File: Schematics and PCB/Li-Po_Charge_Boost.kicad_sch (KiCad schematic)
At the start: 29 parts, among them Q1 FS8205, SW107 Battery Switch, U19 TLV71311PDBVR, U20 TLV70033DDCR, U7 TP4056, U8 MT3608, U9 FS312F-G

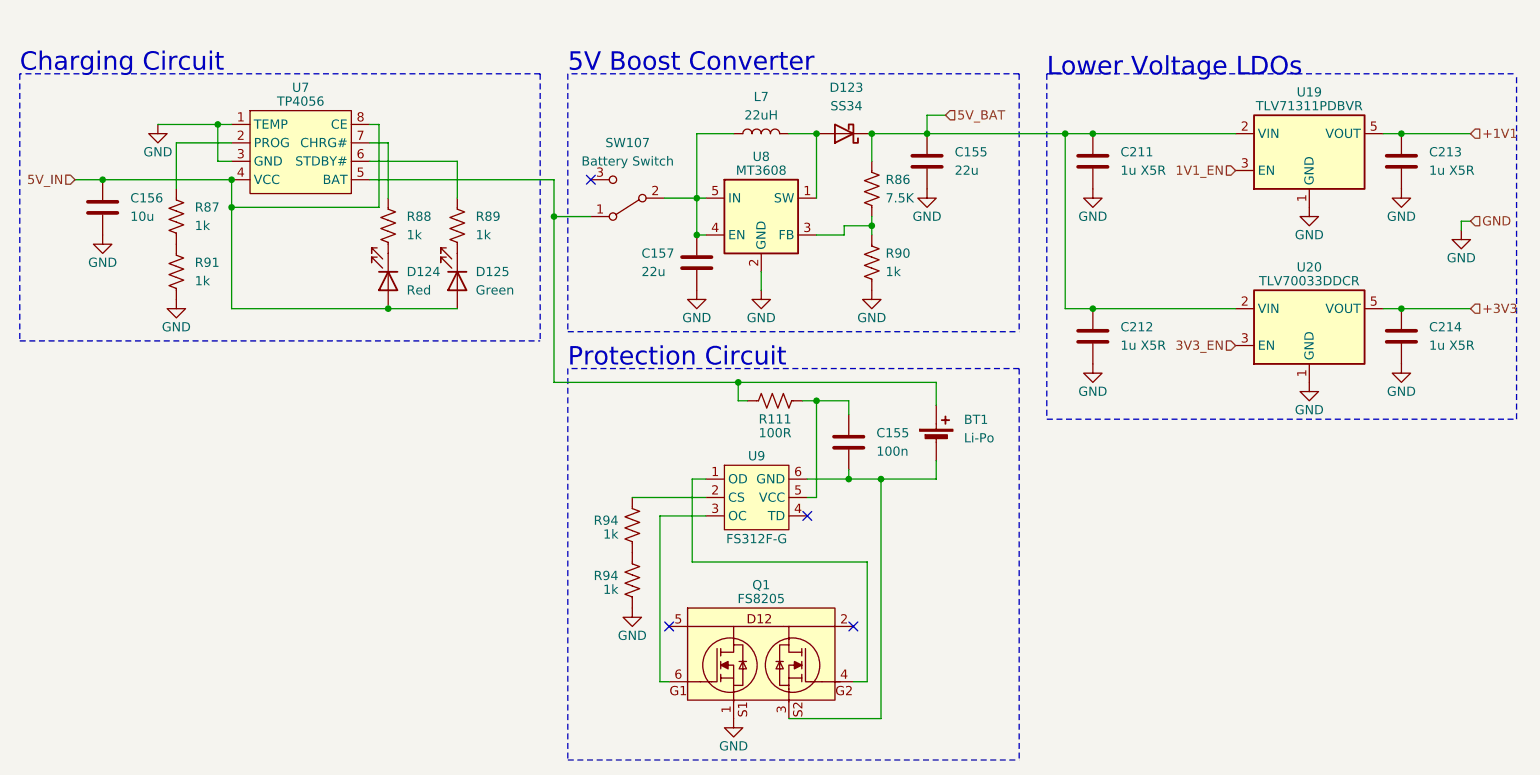
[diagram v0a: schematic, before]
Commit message: minor changes
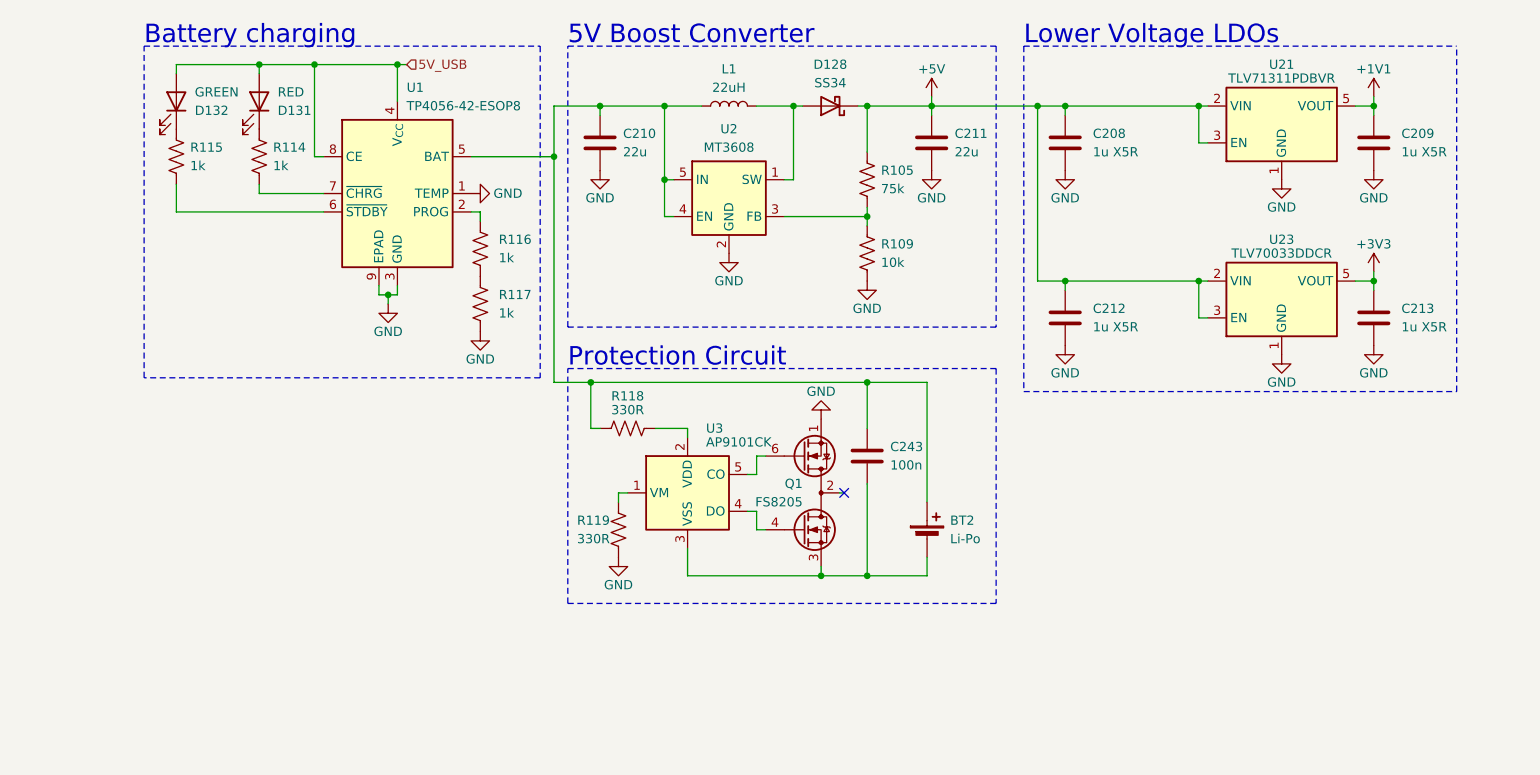
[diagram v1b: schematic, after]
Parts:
- removed BT1: Li-Po, symbol Device:Battery_Cell
- removed C155, C157: 22u, Capacitor_SMD:C_0603_1608Metric, symbol Device:C
- removed C155: 100n, Capacitor_SMD:C_0603_1608Metric, symbol Device:C
- removed C156: 10u, Capacitor_SMD:C_0603_1608Metric, symbol Device:C
- removed D124: Red, LED_SMD:LED_0805_2012Metric, symbol Device:LED
- removed D125: Green, LED_SMD:LED_0805_2012Metric, symbol Device:LED
- removed Q1: FS8205, Package_TO_SOT_SMD:SOT-23-6, symbol Li-Ion Charge Boost Protect:FS8205
- removed R111: 100R, symbol Device:R_US
- removed R87, R88, R89, R91, R94 (x2): 1k, Resistor_SMD:R_0603_1608Metric, symbol Device:R_US
- removed SW107: Battery Switch, Connector_PinHeader_2.54mm:PinHeader_1x03_P2.54mm_Vertical, symbol Switch:SW_SPDT
- removed U7: TP4056, Package_SO:SOP-8-1EP_4.57x4.57mm_P1.27mm_EP4.57x4.45mm_ThermalVias, symbol Li-Ion Charge Boost Protect:TP4056
- removed U8: MT3608, Package_TO_SOT_SMD:SOT-23-6, symbol Regulator_Switching:MT3608
- removed U9: FS312F-G, Package_TO_SOT_SMD:SOT-23-6, symbol Li-Ion Charge Boost Protect:FS312F-G
- added BT2: Li-Po, symbol Device:Battery_Cell
- added C210, C211: 22u, symbol Device:C
- added C243: 100n, Capacitor_SMD:C_0603_1608Metric, symbol Device:C
- added D131: RED, LED_SMD:LED_0805_2012Metric, symbol Device:LED
- added D132: GREEN, LED_SMD:LED_0805_2012Metric, symbol Device:LED
- added Q1: FS8205, Package_TO_SOT_SMD:SOT-23-6, symbol Transistor_FET:DMG9926UDM
- added R114, R115, R116, R117: 1k, Resistor_SMD:R_0603_1608Metric, symbol Device:R_US
- added R118, R119: 330R, Resistor_SMD:R_0603_1608Metric, symbol Device:R_US
- added U1: TP4056-42-ESOP8, Package_SO:SOIC-8-1EP_3.9x4.9mm_P1.27mm_EP2.41x3.3mm_ThermalVias, symbol Battery_Management:TP4056-42-ESOP8
- added U2: MT3608, Package_TO_SOT_SMD:SOT-23-6, symbol Regulator_Switching:MT3608
- added U3: AP9101CK, Package_TO_SOT_SMD:SOT-23-5, symbol Battery_Management:AP9101CK
- R105: renamed from R86; value 7.5K -> 75k
- R109: renamed from R90; value 1k -> 10k
- renumbered C211 to C208, C213 to C209, C214 to C213, D123 to D128, L7 to L1, U19 to U21, U20 to U23
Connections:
- net 3V3_EN is gone; now on net +5V: U23.3 (EN)
- net 5V_BAT is gone; now on net +5V: C208.1, C212.1, D128.1 (K), R105.1, U21.2 (VIN), U23.2 (VIN)
- net GND: now also C210.2, C211.2, Q1.1 (D1), R117.2, R119.2, U1.1 (TEMP), U1.3 (GND), U1.9 (EPAD), U2.2 (GND)
- net at R105.2, R109.1: now also U2.3 (FB)
- net at D128.2 (A), L1.2: now also U2.1 (SW)
- net at L1.1: now also BT2.1 (+), C210.1, C243.2, R118.1, U1.5 (BAT), U2.4 (EN), U2.5 (IN)
- net 1V1_EN renamed +5V
- net +5V: now also C211.1
- new net: R114.1, U1.7 (~{CHRG})
- new net: D131.1 (K), R114.2
- new net: R116.1, U1.2 (PROG)
- new net: R115.1, U1.6 (~{STDBY})
- new net: R118.2, U3.2 (VDD)
- new net: BT2.2 (-), C243.1, Q1.3 (S2), U3.3 (VSS)
- new net: D132.1 (K), R115.2
- new net: R116.2, R117.1
- new net: Q1.2 (S1/D2), Q1.5 (S1/D2)
- new net: Q1.4 (G2), U3.4 (DO)
- new net: Q1.6 (G1), U3.5 (CO)
- new net: R119.1, U3.1 (VM)
- new net 5V_USB: D131.2 (A), D132.2 (A), U1.4 (V_{CC}), U1.8 (CE)
- no-connect marks 4 -> 1
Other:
- note added: "Battery charging"
- note removed: "Charging Circuit"
- moved on the sheet: C208, C209, C212, C213, D128, L1, R105, R109, U21, U23
